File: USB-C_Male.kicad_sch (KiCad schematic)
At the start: 4 parts, among them J1 USB_C_Receptacle_PowerOnly_6P, J2 VBUS, J3 CC, J4 GND

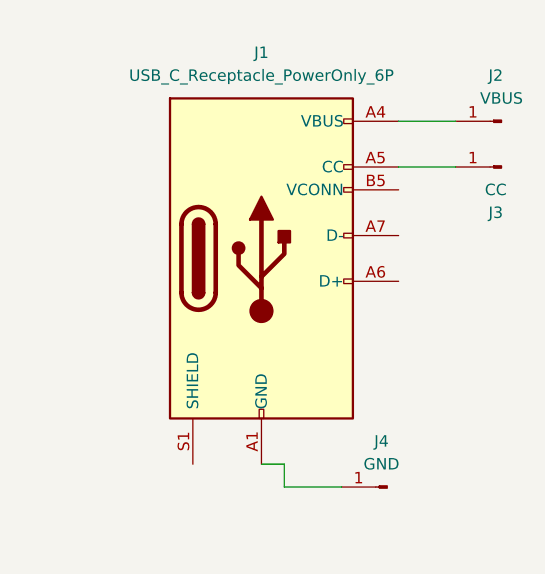
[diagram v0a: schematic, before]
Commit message: nets and fills
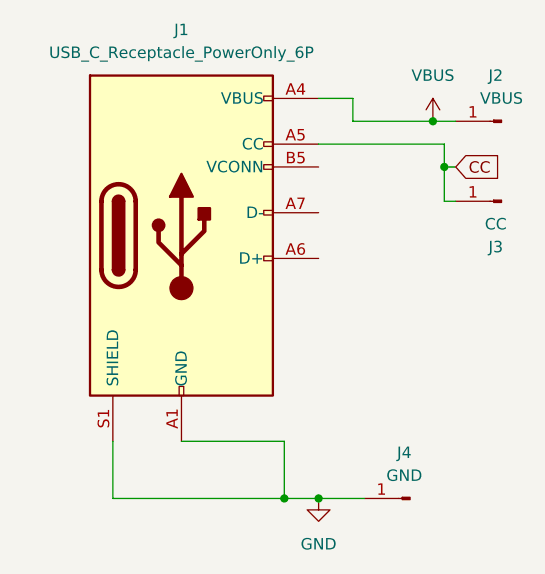
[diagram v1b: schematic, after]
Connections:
- net VBUS: now reaches J1.A4 (VBUS), J1.A9 (VBUS), J1.B4 (VBUS), J1.B9 (VBUS), J2.1 (Pin_1)
- net GND: now reaches J1.A1 (GND), J1.A12 (GND), J1.B1 (GND), J1.B12 (GND), J4.1 (Pin_1)
- net GND: now also J1.S1 (SHIELD)
- net CC: now reaches J1.A5 (CC), J3.1 (Pin_1)
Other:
- moved on the sheet: J1, J3, J4
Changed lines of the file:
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@@
 (kicad_sch (version 20230121) (generator eeschema)
   (paper "A4")
-  (wire (pts (xy 90.17 76.2) (xy 96.52 76.2))
-    (stroke (width 0) (type default))
-  )
-  (wire (pts (xy 77.47 116.84) (xy 77.47 114.3))
-    (stroke (width 0) (type default))
-  )
-  (wire (pts (xy 74.93 114.3) (xy 77.47 114.3))
-    (stroke (width 0) (type default))
-  )
-  (wire (pts (xy 90.17 81.28) (xy 96.52 81.28))
-    (stroke (width 0) (type default))
-  )
-  (wire (pts (xy 83.82 116.84) (xy 77.47 116.84))
-    (stroke (width 0) (type default))
+  (junction (at 77.47 118.11) (diameter 0) (color 0 0 0 0)
+  )
+  (junction (at 93.98 76.2) (diameter 0) (color 0 0 0 0)
+  )
+  (junction (at 81.28 118.11) (diameter 0) (color 0 0 0 0)
+  )
+  (junction (at 95.25 81.28) (diameter 0) (color 0 0 0 0)
+  )
+  (wire (pts (xy 77.47 118.11) (xy 81.28 118.11))
+    (stroke (width 0) (type default))
+  )
+  (wire (pts (xy 77.47 118.11) (xy 77.47 111.76))
+    (stroke (width 0) (type default))
+  )
+  (wire (pts (xy 81.28 73.66) (xy 85.09 73.66))
+    (stroke (width 0) (type default))
+  )
+  (wire (pts (xy 95.25 81.28) (xy 95.25 85.09))
+    (stroke (width 0) (type default))
+  )
+  (wire (pts (xy 93.98 76.2) (xy 96.52 76.2))
+    (stroke (width 0) (type default))
+  )
+  (wire (pts (xy 95.25 78.74) (xy 95.25 81.28))
+    (stroke (width 0) (type default))
+  )
+  (wire (pts (xy 66.04 111.76) (xy 77.47 111.76))
+    (stroke (width 0) (type default))
+  )
+  (wire (pts (xy 95.25 85.09) (xy 96.52 85.09))
+    (stroke (width 0) (type default))
+  )
+  (wire (pts (xy 96.52 81.28) (xy 95.25 81.28))
+    (stroke (width 0) (type default))
+  )
+  (wire (pts (xy 85.09 73.66) (xy 85.09 76.2))
+    (stroke (width 0) (type default))
+  )
+  (wire (pts (xy 58.42 111.76) (xy 58.42 118.11))
+    (stroke (width 0) (type default))
+  )
+  (wire (pts (xy 58.42 118.11) (xy 77.47 118.11))
+    (stroke (width 0) (type default))
+  )
+  (wire (pts (xy 85.09 76.2) (xy 93.98 76.2))
+    (stroke (width 0) (type default))
+  )
+  (wire (pts (xy 81.28 118.11) (xy 86.36 118.11))
+    (stroke (width 0) (type default))
+  )
+  (wire (pts (xy 81.28 78.74) (xy 95.25 78.74))
+    (stroke (width 0) (type default))
+  )
+  (global_label "CC" (shape input) (at 96.52 81.28 0) (fields_autoplaced)
+    (effects (font (size 1.27 1.27)) (justify left))
+    (property "Intersheetrefs" "${INTERSHEET_REFS}" (at 102.0452 81.28 0)
+      (effects (font (size 1.27 1.27)) (justify left) hide)
+    )
   )
   (symbol (lib_id "Connector:Conn_01x01_Pin") (at 101.6 76.2 0) (mirror y) (unit 1)
@@
     )
   )
-  (symbol (lib_id "Connector:USB_C_Plug_USB2.0") (at 74.93 91.44 0) (unit 1)
-    (in_bom yes) (on_board yes) (dnp no) (fields_autoplaced)
-    (property "Reference" "J1" (at 74.93 68.58 0)
-      (effects (font (size 1.27 1.27)))
-    )
-    (property "Value" "USB_C_Receptacle_PowerOnly_6P" (at 74.93 71.12 0)
-      (effects (font (size 1.27 1.27)))
-    )
-    (property "Footprint" "Connector_USB:USB_C_Plug_JAE_DX07P024AJ1" (at 78.74 91.44 0)
-      (effects (font (size 1.27 1.27)) hide)
-    )
-    (property "Datasheet" "https://www.usb.org/sites/default/files/documents/usb_type-c.zip" (at 78.74 91.44 0)
+  (symbol (lib_id "Connector:USB_C_Plug_USB2.0") (at 66.04 88.9 0) (unit 1)
+    (in_bom yes) (on_board yes) (dnp no) (fields_autoplaced)
+    (property "Reference" "J1" (at 66.04 66.04 0)
+      (effects (font (size 1.27 1.27)))
+    )
+    (property "Value" "USB_C_Receptacle_PowerOnly_6P" (at 66.04 68.58 0)
+      (effects (font (size 1.27 1.27)))
+    )
+    (property "Footprint" "Connector_USB:USB_C_Plug_JAE_DX07P024AJ1" (at 69.85 88.9 0)
+      (effects (font (size 1.27 1.27)) hide)
+    )
+    (property "Datasheet" "https://www.usb.org/sites/default/files/documents/usb_type-c.zip" (at 69.85 88.9 0)
       (effects (font (size 1.27 1.27)) hide)
     )
@@
     )
   )
-  (symbol (lib_name "Conn_01x01_Pin_1") (lib_id "Connector:Conn_01x01_Pin") (at 101.6 81.28 0) (mirror y) (unit 1)
-    (in_bom yes) (on_board yes) (dnp no) (fields_autoplaced)
-    (property "Reference" "J3" (at 100.965 86.36 0)
-      (effects (font (size 1.27 1.27)))
-    )
-    (property "Value" "CC" (at 100.965 83.82 0)
-      (effects (font (size 1.27 1.27)))
-    )
-    (property "Footprint" "TestPoint:TestPoint_Pad_2.0x2.0mm" (at 101.6 81.28 0)
-      (effects (font (size 1.27 1.27)) hide)
-    )
-    (property "Datasheet" "~" (at 101.6 81.28 0)
+  (symbol (lib_id "power:VBUS") (at 93.98 76.2 0) (unit 1)
+    (in_bom yes) (on_board yes) (dnp no) (fields_autoplaced)
+    (property "Reference" "#PWR01" (at 93.98 80.01 0)
+      (effects (font (size 1.27 1.27)) hide)
+    )
+    (property "Value" "VBUS" (at 93.98 71.12 0)
+      (effects (font (size 1.27 1.27)))
+    )
+    (property "Footprint" "" (at 93.98 76.2 0)
+      (effects (font (size 1.27 1.27)) hide)
+    )
+    (property "Datasheet" "" (at 93.98 76.2 0)
+      (effects (font (size 1.27 1.27)) hide)
+    )
+    (pin "1")
+    (instances
+      (project "USB-C_Male"
+        (path "/63a59359-4c09-4b05-9530-0121e3690278"
+          (reference "#PWR01") (unit 1)
+        )
+      )
+    )
+  )
+  (symbol (lib_id "power:GND") (at 81.28 118.11 0) (unit 1)
+    (in_bom yes) (on_board yes) (dnp no) (fields_autoplaced)
+    (property "Reference" "#PWR02" (at 81.28 124.46 0)
+      (effects (font (size 1.27 1.27)) hide)
+    )
+    (property "Value" "GND" (at 81.28 123.19 0)
+      (effects (font (size 1.27 1.27)))
+    )
+    (property "Footprint" "" (at 81.28 118.11 0)
+      (effects (font (size 1.27 1.27)) hide)
+    )
+    (property "Datasheet" "" (at 81.28 118.11 0)
+      (effects (font (size 1.27 1.27)) hide)
+    )
+    (pin "1")
+    (instances
+      (project "USB-C_Male"
+        (path "/63a59359-4c09-4b05-9530-0121e3690278"
+          (reference "#PWR02") (unit 1)
+        )
+      )
+    )
+  )
+  (symbol (lib_name "Conn_01x01_Pin_1") (lib_id "Connector:Conn_01x01_Pin") (at 101.6 85.09 0) (mirror y) (unit 1)
+    (in_bom yes) (on_board yes) (dnp no) (fields_autoplaced)
+    (property "Reference" "J3" (at 100.965 90.17 0)
+      (effects (font (size 1.27 1.27)))
+    )
+    (property "Value" "CC" (at 100.965 87.63 0)
+      (effects (font (size 1.27 1.27)))
+    )
+    (property "Footprint" "TestPoint:TestPoint_Pad_2.0x2.0mm" (at 101.6 85.09 0)
+      (effects (font (size 1.27 1.27)) hide)
+    )
+    (property "Datasheet" "~" (at 101.6 85.09 0)
       (effects (font (size 1.27 1.27)) hide)
     )
@@
     )
   )
-  (symbol (lib_id "Connector:Conn_01x01_Pin") (at 88.9 116.84 0) (mirror y) (unit 1)
+  (symbol (lib_id "Connector:Conn_01x01_Pin") (at 91.44 118.11 0) (mirror y) (unit 1)
     (in_bom yes) (on_board yes) (dnp no)
-    (property "Reference" "J4" (at 88.265 111.76 0)
-      (effects (font (size 1.27 1.27)))
-    )
-    (property "Value" "GND" (at 88.265 114.3 0)
-      (effects (font (size 1.27 1.27)))
-    )
-    (property "Footprint" "TestPoint:TestPoint_Pad_2.0x2.0mm" (at 88.9 116.84 0)
-      (effects (font (size 1.27 1.27)) hide)
-    )
-    (property "Datasheet" "~" (at 88.9 116.84 0)
-      (effects (font (size 1.27 1.27)) hide)
-    )
+    (property "Reference" "J4" (at 90.805 113.03 0)
+      (effects (font (size 1.27 1.27)))
+    )
+    (property "Value" "GND" (at 90.805 115.57 0)
+      (effects (font (size 1.27 1.27)))
+    )
+    (property "Footprint" "TestPoint:TestPoint_Pad_2.0x2.0mm" (at 91.44 118.11 0)
+      (effects (font (size 1.27 1.27)) hide)
+    )
+    (property "Datasheet" "~" (at 91.44 118.11 0)
+      (effects (font (size 1.27 1.27)) hide)
+    )
